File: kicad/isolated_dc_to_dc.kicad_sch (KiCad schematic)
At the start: 7 parts, among them U5 LM25184NGUR, U6 750313445

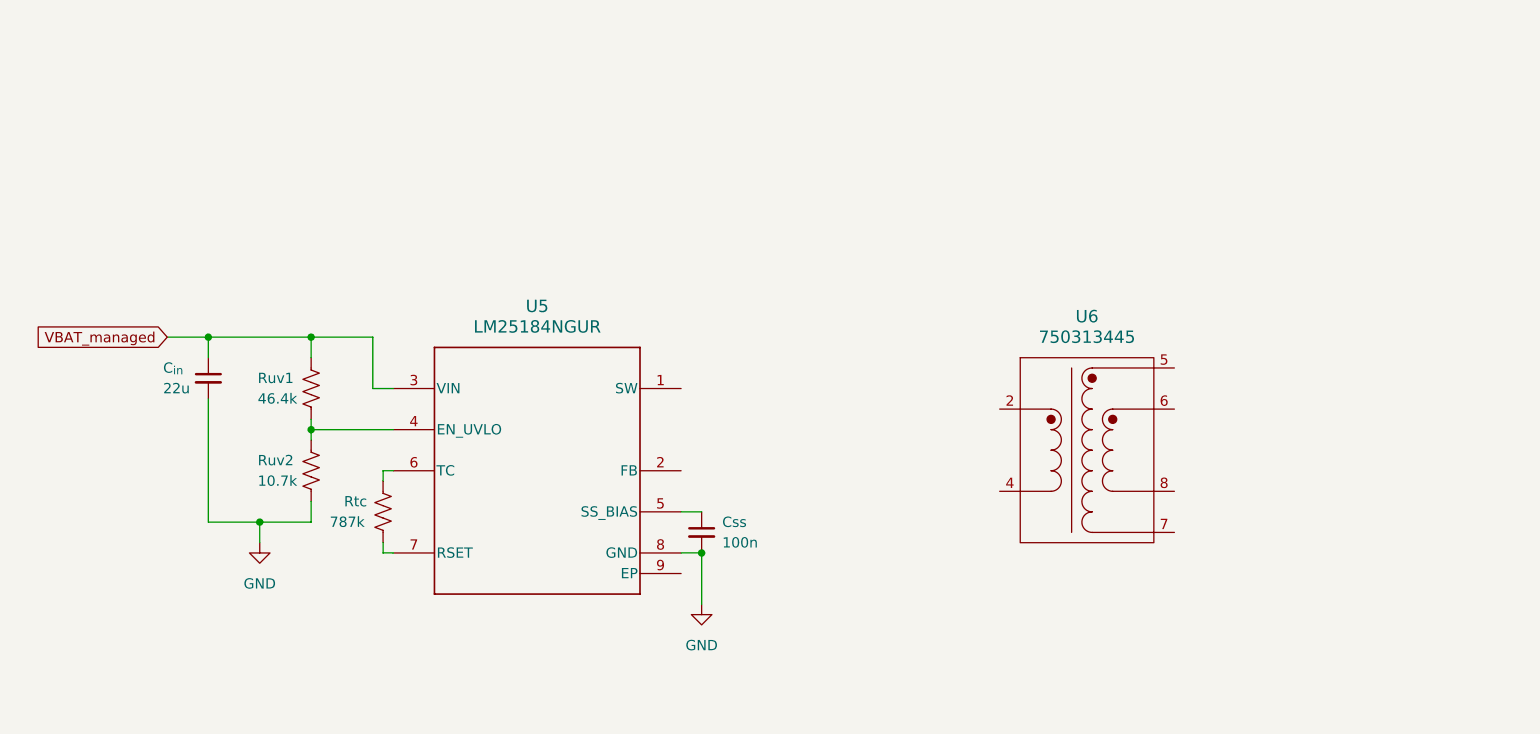
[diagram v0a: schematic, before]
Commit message: kicad
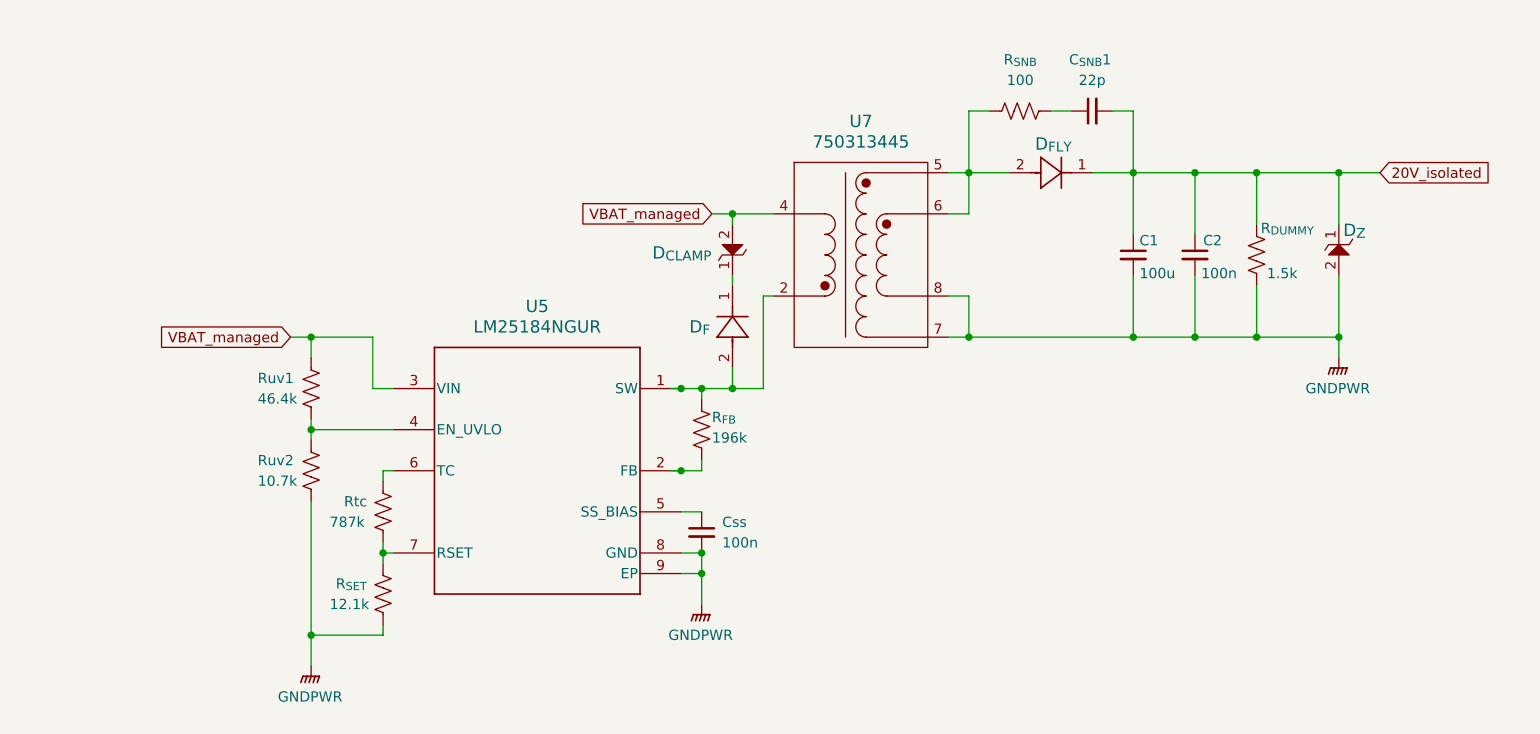
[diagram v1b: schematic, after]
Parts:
- removed C_{in}: 22u, symbol Device:C_Small
- removed U6: 750313445, SOIC_13445_WRE, symbol transformer_750313445:750313445
- added C1: 100u, symbol Device:C_Small
- added C2: 100n, symbol Device:C_Small
- added C_{SNB}1: 22p, symbol Device:C_Small
- added D_{CLAMP}, D_{Z}: PDZVTR9.1B, DIO_PDZVTFT_ROM, symbol zener_PDZVTR9.1B:PDZVTR9.1B
- added D_{FLY}, D_{F}: SK510A-LTP, SMADO-214AC_LEAD-FRAME_MCC, symbol schottky_SK510A-LTP:SK510A-LTP
- added R_{DUMMY}: 1.5k, symbol Device:R_US
- added R_{FB}: 196k, symbol Device:R_US
- added R_{SET}: 12.1k, symbol Device:R_US
- added R_{SNB}: 100, symbol Device:R_US
- added U7: 750313445, SOIC_13445_WRE, symbol transformer_750313445:750313445
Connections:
- net GND is gone; now on net GNDPWR: Css.2, Ruv2.2, U5.8 (GND)
- net VBAT_managed: now also D_{CLAMP}.2, U7.4
- net at Rtc.2, U5.7 (RSET): now also R_{SET}.1
- net at U5.1 (SW): now also D_{F}.2, R_{FB}.1, U7.2
- net at U5.2 (FB): now also R_{FB}.2
- net GNDPWR: now reaches U5.9 (EP)
- net GNDPWR: now also C1.2, C2.2, D_{Z}.2, R_{DUMMY}.1, R_{SET}.2, U7.7, U7.8
- new net: D_{FLY}.2, R_{SNB}.1, U7.5, U7.6
- new net: C_{SNB}1.1, R_{SNB}.2
- new net: D_{CLAMP}.1, D_{F}.1
- new net 20V_isolated: C1.1, C2.1, C_{SNB}1.2, D_{FLY}.1, D_{Z}.1, R_{DUMMY}.2

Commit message: kicad
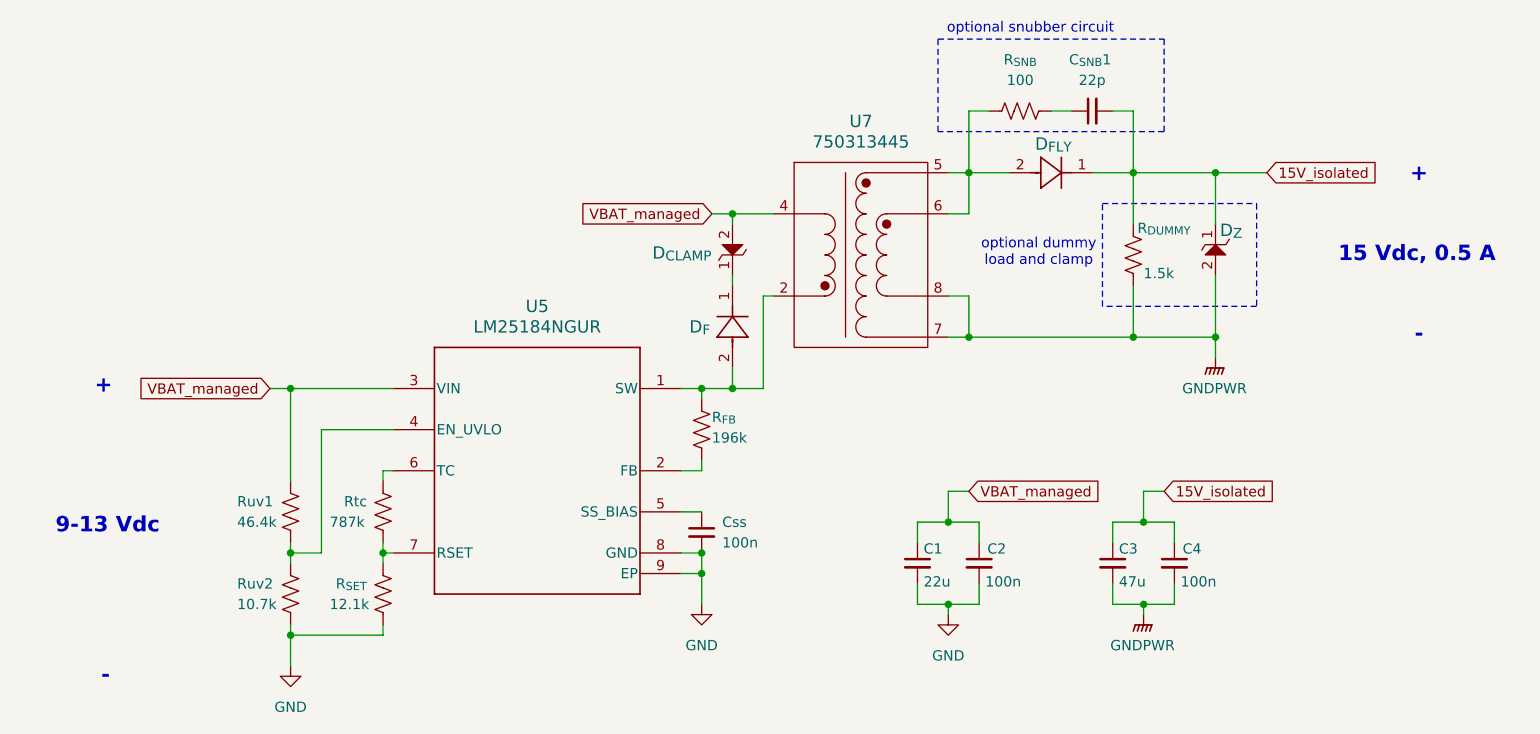
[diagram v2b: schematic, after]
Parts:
- added C3: 47u, symbol Device:C_Small
- added C4: 100n, symbol Device:C_Small
- C1: value 100u -> 22u
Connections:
- net GNDPWR: now also C3.2, C4.2; no longer C1.2, C2.2, Css.2, R_{SET}.2, Ruv2.2, U5.8 (GND), U5.9 (EP)
- net VBAT_managed: now also C1.1, C2.1
- net 20V_isolated renamed 15V_isolated
- net 15V_isolated: now also C3.1, C4.1; no longer C1.1, C2.1
- new net GND: C1.2, C2.2, Css.2, R_{SET}.2, Ruv2.2, U5.8 (GND), U5.9 (EP)
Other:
- note added: "+"
- note added: "-"
- note added: "15 Vdc, 0.5 A"
- note added: "9-13 Vdc"
- note added: "optional dummy load and clamp"
- note added: "optional snubber circuit"
- moved on the sheet: C1, C2, D_{Z}, R_{DUMMY}, Ruv1, Ruv2
